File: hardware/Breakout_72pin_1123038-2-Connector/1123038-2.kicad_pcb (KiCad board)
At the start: 2 copper layers, 77.5 x 33.7 mm, 16 parts, among them P1 CONN_1, P10 1123038-2, P11 CONN_01X05, P12 CONN_01X05, P13 CONN_01X08, P14 CONN_01X06, P15 CONN_01X05, P2 CONN_1, P3 CONN_01X05, P4 CONN_01X06, P5 CONN_01X06, P6 CONN_01X05, P7 CONN_01X08, P8 CONN_01X08, P9 CONN_01X05

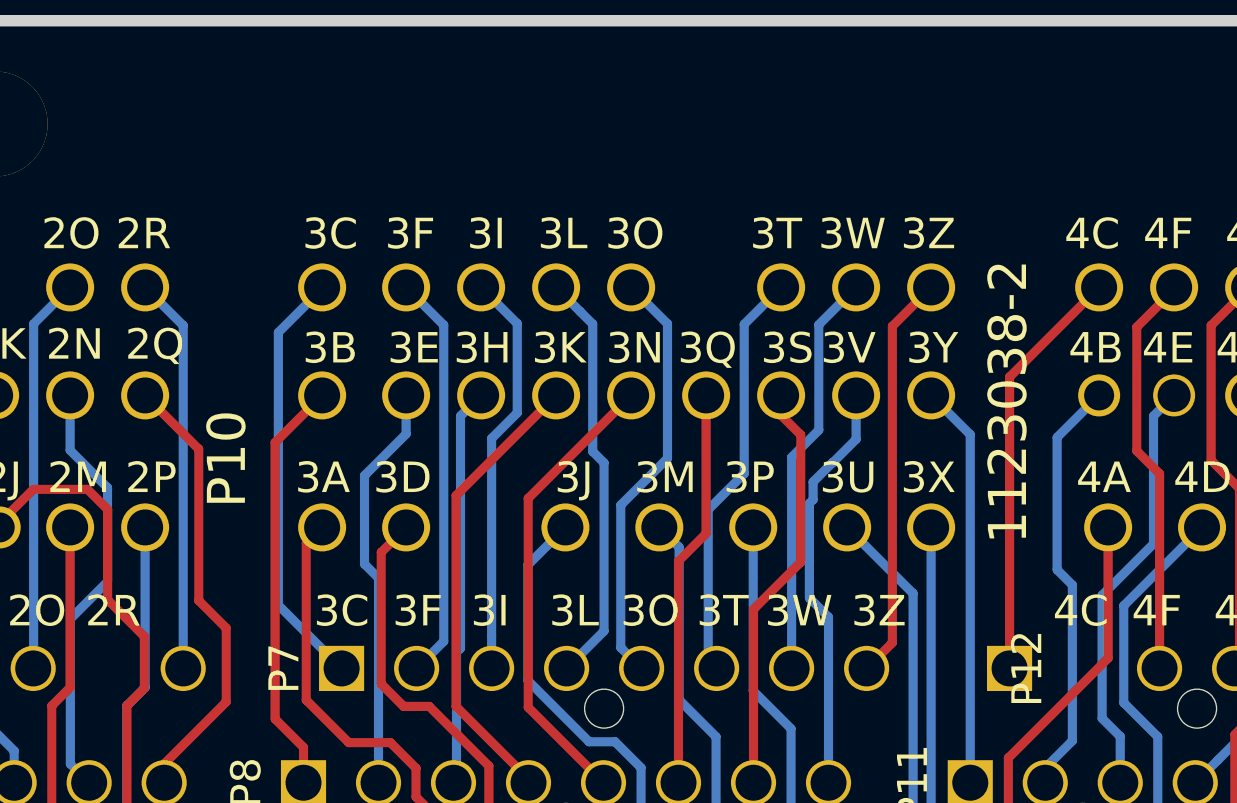
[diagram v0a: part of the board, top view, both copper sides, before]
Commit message: update pcb files
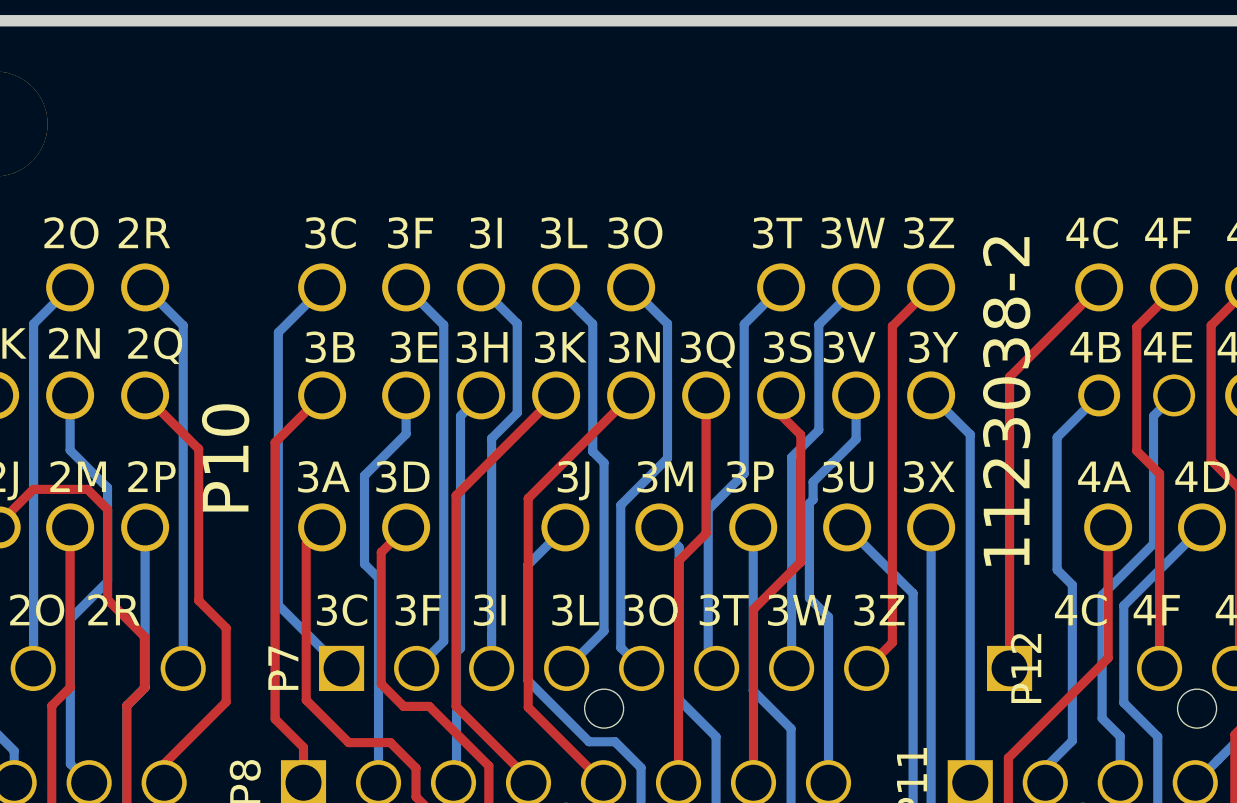
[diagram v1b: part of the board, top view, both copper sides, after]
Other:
- net class 1.5A removed
- net class 10A removed
- net class Default removed
